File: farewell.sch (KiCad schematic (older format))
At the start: 27 parts, among them U1 0

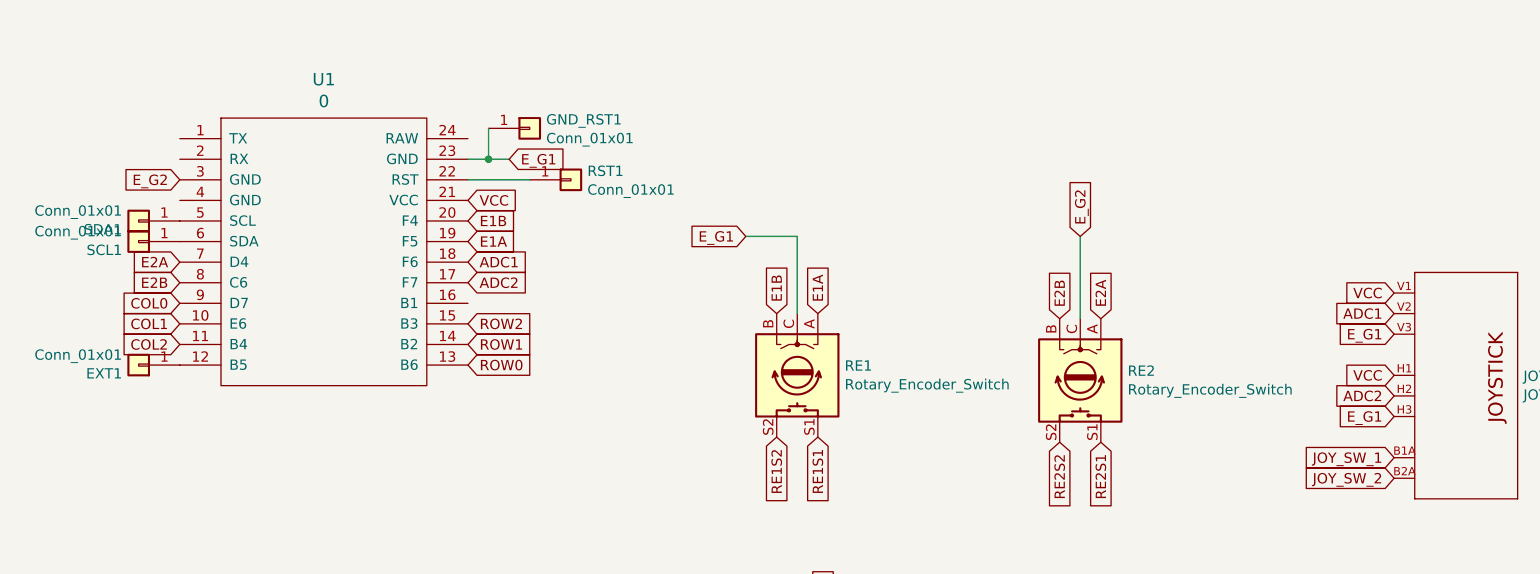
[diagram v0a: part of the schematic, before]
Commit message: farewell v1 pcb
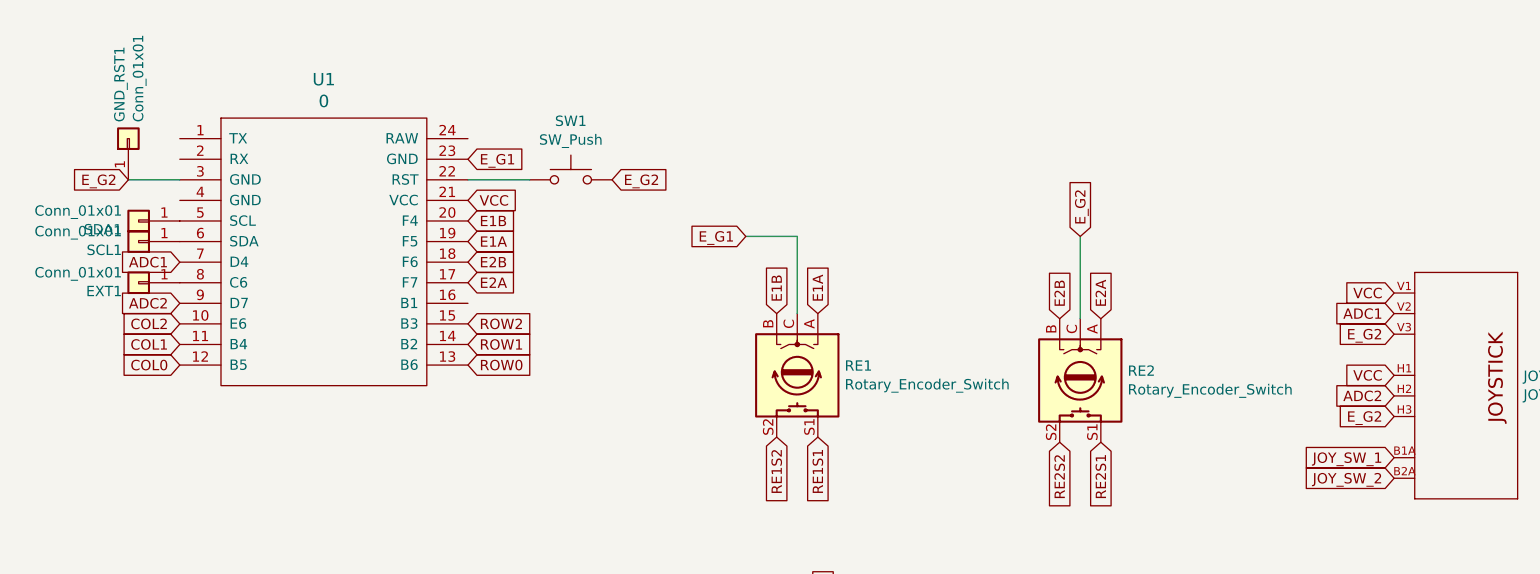
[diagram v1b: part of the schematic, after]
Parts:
- removed RST1: Conn_01x01, pin:Pin_D0.7mm_L6.5mm_W1.8mm_FlatFork, symbol Connector_Generic:Conn_01x01
- added SW1: SW_Push, random-kb-part:PushButton_6x6mm_TH_Pretty, symbol Switch:SW_Push
- EXT1, GND_RST1, SCL1, SDA1: footprint pin:Pin_D0.7mm_L6.5mm_W1.8mm_FlatFork -> keyboard_parts:PIN_1
- JOY1: footprint JOYSTICK -> sparkfun-electromech:JOYSTICK
- MX1, MX2, MX3, MX4, MX5, MX6, MX7, MX8, MX9: footprint MX_Alps_Hybrid:MX-1U-NoLED -> farewell:MX-1U-NoLED-NoPCBMount
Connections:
- net ADC1: now also U1.7 (D4); no longer U1.18 (F6)
- net ADC2: now also U1.9 (D7); no longer U1.17 (F7)
- net COL0: now also U1.12 (B5); no longer U1.9 (D7)
- net COL1: now also U1.11 (B4); no longer U1.10 (E6)
- net COL2: now also U1.10 (E6); no longer U1.11 (B4)
- net E2A: now also U1.17 (F7); no longer U1.7 (D4)
- net E2B: now also U1.18 (F6); no longer U1.8 (C6)
- net E_G1: no longer GND_RST1.1 (Pin_1), JOY1.H3 (H-), JOY1.V3 (V-)
- net E_G2: now also GND_RST1.1 (Pin_1), JOY1.H3 (H-), JOY1.V3 (V-), SW1.2
- net at U1.22 (RST): now also SW1.1
- net at EXT1.1 (Pin_1): now also U1.8 (C6); no longer U1.12 (B5)
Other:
- moved on the sheet: EXT1, GND_RST1
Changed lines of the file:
@@
 F 0 "MX1" H 3061 6892 60  0000 C CNN
 F 1 "MX-1U" H 3061 6818 20  0000 C CNN
-F 2 "MX_Alps_Hybrid:MX-1U-NoLED" H 2950 6650 60  0001 C CNN
+F 2 "farewell:MX-1U-NoLED-NoPCBMount" H 2950 6650 60  0001 C CNN
 F 3 "" H 2950 6650 60  0001 C CNN
 	1    2975 6675
@@
 F 0 "MX2" H 4011 6892 60  0000 C CNN
 F 1 "MX-1U" H 4011 6818 20  0000 C CNN
-F 2 "MX_Alps_Hybrid:MX-1U-NoLED" H 3900 6650 60  0001 C CNN
+F 2 "farewell:MX-1U-NoLED-NoPCBMount" H 3900 6650 60  0001 C CNN
 F 3 "" H 3900 6650 60  0001 C CNN
 	1    3925 6675
@@
 F 0 "MX3" H 5061 6892 60  0000 C CNN
 F 1 "MX-1U" H 5061 6818 20  0000 C CNN
-F 2 "MX_Alps_Hybrid:MX-1U-NoLED" H 4950 6650 60  0001 C CNN
+F 2 "farewell:MX-1U-NoLED-NoPCBMount" H 4950 6650 60  0001 C CNN
 F 3 "" H 4950 6650 60  0001 C CNN
 	1    4975 6675
@@
 F 0 "MX4" H 3061 6017 60  0000 C CNN
 F 1 "MX-1U" H 3061 5943 20  0000 C CNN
-F 2 "MX_Alps_Hybrid:MX-1U-NoLED" H 2950 5775 60  0001 C CNN
+F 2 "farewell:MX-1U-NoLED-NoPCBMount" H 2950 5775 60  0001 C CNN
 F 3 "" H 2950 5775 60  0001 C CNN
 	1    2975 5800
@@
 F 0 "MX5" H 4011 6017 60  0000 C CNN
 F 1 "MX-1U" H 4011 5943 20  0000 C CNN
-F 2 "MX_Alps_Hybrid:MX-1U-NoLED" H 3900 5775 60  0001 C CNN
+F 2 "farewell:MX-1U-NoLED-NoPCBMount" H 3900 5775 60  0001 C CNN
 F 3 "" H 3900 5775 60  0001 C CNN
 	1    3925 5800
@@
 F 0 "MX6" H 5061 6017 60  0000 C CNN
 F 1 "MX-1U" H 5061 5943 20  0000 C CNN
-F 2 "MX_Alps_Hybrid:MX-1U-NoLED" H 4950 5775 60  0001 C CNN
+F 2 "farewell:MX-1U-NoLED-NoPCBMount" H 4950 5775 60  0001 C CNN
 F 3 "" H 4950 5775 60  0001 C CNN
 	1    4975 5800
@@
 F 0 "MX7" H 3061 5017 60  0000 C CNN
 F 1 "MX-1U" H 3061 4943 20  0000 C CNN
-F 2 "MX_Alps_Hybrid:MX-1U-NoLED" H 2950 4775 60  0001 C CNN
+F 2 "farewell:MX-1U-NoLED-NoPCBMount" H 2950 4775 60  0001 C CNN
 F 3 "" H 2950 4775 60  0001 C CNN
 	1    2975 4800
@@
 F 0 "MX8" H 4011 4992 60  0000 C CNN
 F 1 "MX-1U" H 4011 4918 20  0000 C CNN
-F 2 "MX_Alps_Hybrid:MX-1U-NoLED" H 3900 4750 60  0001 C CNN
+F 2 "farewell:MX-1U-NoLED-NoPCBMount" H 3900 4750 60  0001 C CNN
 F 3 "" H 3900 4750 60  0001 C CNN
 	1    3925 4775
@@
 F 0 "MX9" H 5061 4967 60  0000 C CNN
 F 1 "MX-1U" H 5061 4893 20  0000 C CNN
-F 2 "MX_Alps_Hybrid:MX-1U-NoLED" H 4950 4725 60  0001 C CNN
+F 2 "farewell:MX-1U-NoLED-NoPCBMount" H 4950 4725 60  0001 C CNN
 F 3 "" H 4950 4725 60  0001 C CNN
 	1    4975 4750
@@
 Wire Wire Line
 	4100 2125 4100 2500
-Text GLabel 2700 1750 2    50   Input ~ 0
-E_G1
-Text GLabel 1100 2250 0    50   Input ~ 0
+Text GLabel 2500 2350 2    50   Input ~ 0
 E2A
-Text GLabel 1100 2350 0    50   Input ~ 0
+Text GLabel 2500 2250 2    50   Input ~ 0
 E2B
 Text GLabel 2500 2150 2    50   Input ~ 0
@@
 Text GLabel 5275 4250 2    50   Input ~ 0
 RE2S2
+Text GLabel 1100 2550 0    50   Input ~ 0
+COL2
 Text GLabel 1100 2650 0    50   Input ~ 0
-COL2
-Text GLabel 1100 2550 0    50   Input ~ 0
 COL1
-Text GLabel 1100 2450 0    50   Input ~ 0
+Text GLabel 1100 2750 0    50   Input ~ 0
 COL0
 Text GLabel 5475 2125 1    50   Input ~ 0
 E_G2
-Text GLabel 1100 1850 0    50   Input ~ 0
+Text GLabel 850  1850 0    50   Input ~ 0
 E_G2
 Wire Wire Line
@@
 Wire Wire Line
 	2675 5375 3625 5375
-Wire Wire Line
-	2500 1750 2600 1750
-$Comp
-L Connector_Generic:Conn_01x01 RST1
-U 1 1 5CA633F3
-P 3000 1850
-F 0 "RST1" H 3080 1892 50  0000 L CNN
-F 1 "Conn_01x01" H 3080 1801 50  0000 L CNN
-F 2 "pin:Pin_D0.7mm_L6.5mm_W1.8mm_FlatFork" H 3000 1850 50  0001 C CNN
-F 3 "~" H 3000 1850 50  0001 C CNN
-	1    3000 1850
-	1    0    0    -1
-$EndComp
 $Comp
 L Connector_Generic:Conn_01x01 GND_RST1
 U 1 1 5CA6404D
-P 2800 1600
-F 0 "GND_RST1" H 2880 1642 50  0000 L CNN
-F 1 "Conn_01x01" H 2880 1551 50  0000 L CNN
-F 2 "pin:Pin_D0.7mm_L6.5mm_W1.8mm_FlatFork" H 2800 1600 50  0001 C CNN
-F 3 "~" H 2800 1600 50  0001 C CNN
-	1    2800 1600
-	1    0    0    -1
+P 850 1650
+F 0 "GND_RST1" H 930 1692 50  0000 L CNN
+F 1 "Conn_01x01" H 930 1601 50  0000 L CNN
+F 2 "keyboard_parts:PIN_1" H 850 1650 50  0001 C CNN
+F 3 "~" H 850 1650 50  0001 C CNN
+	1    850  1650
+	0    -1   -1   0
 $EndComp
 Wire Wire Line
 	2800 1850 2500 1850
-Wire Wire Line
-	2600 1750 2600 1600
-Connection ~ 2600 1750
-Wire Wire Line
-	2600 1750 2700 1750
 $Comp
 L sparkfun-electromech:JOYSTICKPTH JOY1
@@
 F 0 "JOY1" H 7628 2796 50  0000 L CNN
 F 1 "JOYSTICKPTH" H 7628 2705 50  0000 L CNN
-F 2 "JOYSTICK" H 7430 2950 20  0001 C CNN
+F 2 "sparkfun-electromech:JOYSTICK" H 7430 2950 20  0001 C CNN
 F 3 "" H 7400 2800 50  0001 C CNN
 	1    7400 2800
@@
 F 0 "SCL1" H 980 2192 50  0000 L CNN
 F 1 "Conn_01x01" H 980 2101 50  0000 L CNN
-F 2 "pin:Pin_D0.7mm_L6.5mm_W1.8mm_FlatFork" H 900 2150 50  0001 C CNN
+F 2 "keyboard_parts:PIN_1" H 900 2150 50  0001 C CNN
 F 3 "~" H 900 2150 50  0001 C CNN
 	1    900  2150
@@
 F 0 "SDA1" H 980 2092 50  0000 L CNN
 F 1 "Conn_01x01" H 980 2001 50  0000 L CNN
-F 2 "pin:Pin_D0.7mm_L6.5mm_W1.8mm_FlatFork" H 900 2050 50  0001 C CNN
+F 2 "keyboard_parts:PIN_1" H 900 2050 50  0001 C CNN
 F 3 "~" H 900 2050 50  0001 C CNN
 	1    900  2050
@@
 L Connector_Generic:Conn_01x01 EXT1
 U 1 1 5CAA7D24
-P 900 2750
-F 0 "EXT1" H 980 2792 50  0000 L CNN
-F 1 "Conn_01x01" H 980 2701 50  0000 L CNN
-F 2 "pin:Pin_D0.7mm_L6.5mm_W1.8mm_FlatFork" H 900 2750 50  0001 C CNN
-F 3 "~" H 900 2750 50  0001 C CNN
-	1    900  2750
+P 900 2350
+F 0 "EXT1" H 980 2392 50  0000 L CNN
+F 1 "Conn_01x01" H 980 2301 50  0000 L CNN
+F 2 "keyboard_parts:PIN_1" H 900 2350 50  0001 C CNN
+F 3 "~" H 900 2350 50  0001 C CNN
+	1    900  2350
 	-1   0    0    1
 $EndComp
-Text GLabel 2500 2250 2    50   Input ~ 0
+Text GLabel 1100 2250 0    50   Input ~ 0
 ADC1
-Text GLabel 2500 2350 2    50   Input ~ 0
+Text GLabel 1100 2450 0    50   Input ~ 0
 ADC2
 Text GLabel 2500 1950 2    50   Input ~ 0
@@
 VCC
 Text GLabel 7000 2600 0    50   Input ~ 0
-E_G1
+E_G2
 Text GLabel 7000 3000 0    50   Input ~ 0
-E_G1
+E_G2
 Text GLabel 7000 2500 0    50   Input ~ 0
 ADC1
@@
 Text GLabel 4225 4300 2    50   Input ~ 0
 JOY_SW_2
+Wire Wire Line
+	1100 1850 850  1850
+Text GLabel 2500 1750 2    50   Input ~ 0
+E_G1
+$Comp
+L Switch:SW_Push SW1
+U 1 1 5CB34881
+P 3000 1850
+F 0 "SW1" H 3000 2135 50  0000 C CNN
+F 1 "SW_Push" H 3000 2044 50  0000 C CNN
+F 2 "random-kb-part:PushButton_6x6mm_TH_Pretty" H 3000 2050 50  0001 C CNN
+F 3 "~" H 3000 2050 50  0001 C CNN
+	1    3000 1850
+	1    0    0    -1
+$EndComp
+Text GLabel 3200 1850 2    50   Input ~ 0
+E_G2
 $EndSCHEMATC
